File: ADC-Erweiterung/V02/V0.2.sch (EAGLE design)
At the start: 32 parts, among them IC101 ADS124S06IPBS, X101 MOLEX-8738-0343, X102 A97581-ND, X103 A97581-ND, X104 A97581-ND, X105 33PIN-2.54

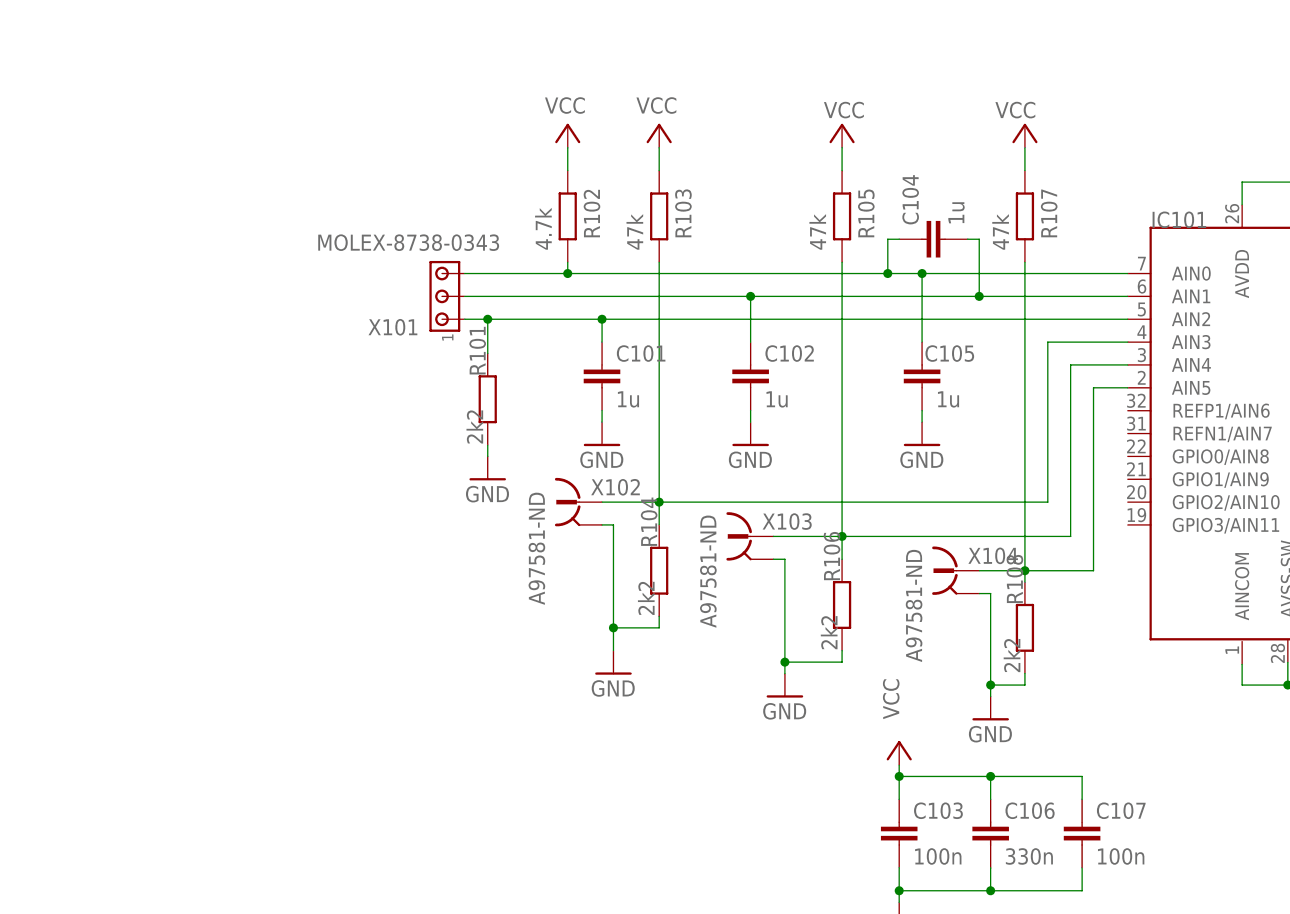
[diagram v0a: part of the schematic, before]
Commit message: AbgabeSoftware
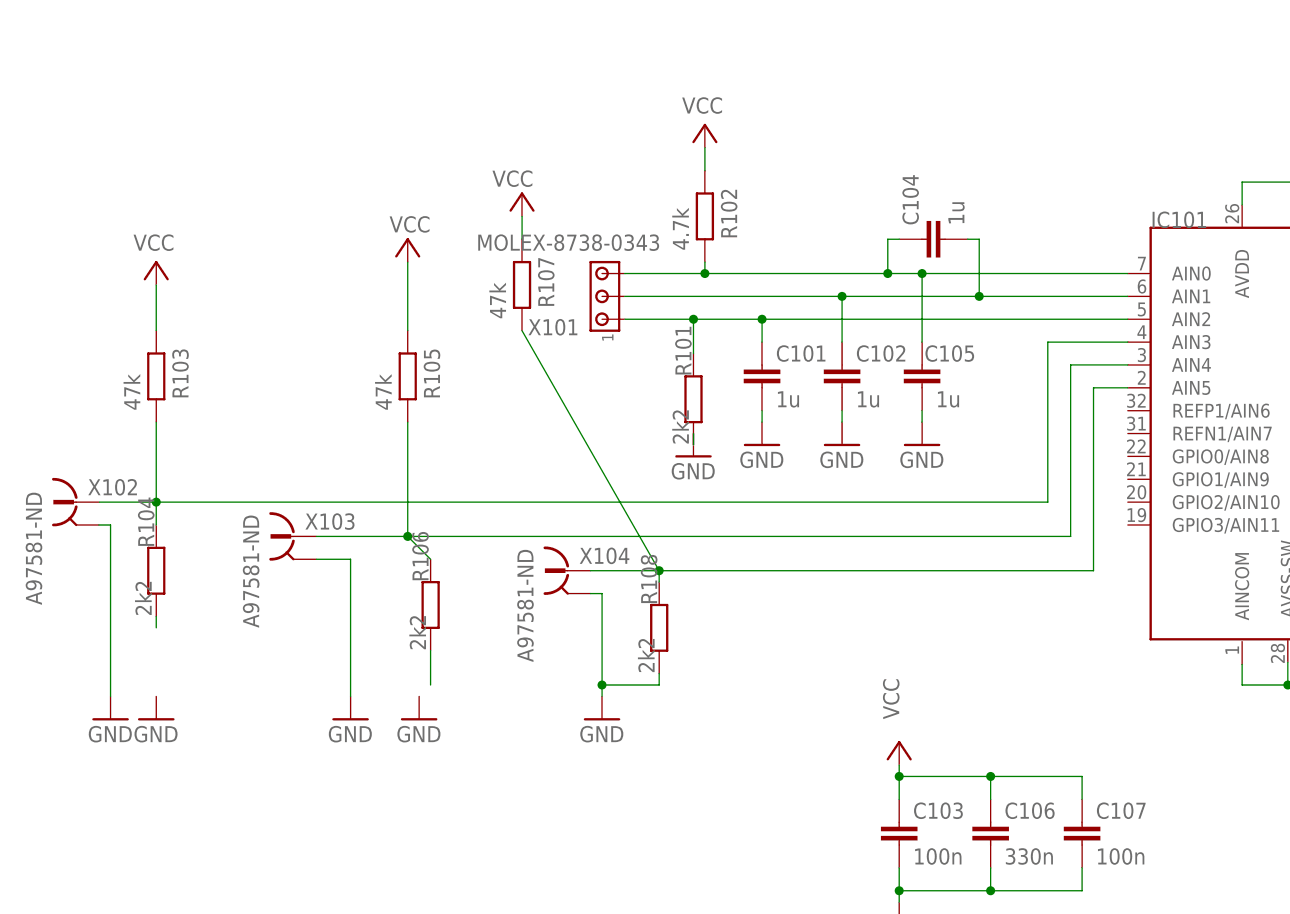
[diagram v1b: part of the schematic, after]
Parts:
- SV101: DIGIKEY_NR (none) -> 732-5321-ND; DIGIKEY_PRICE (none) -> 0.37
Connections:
- new net N$8: R104.1
- new net N$9: R106.1
- net GND: no longer R104.1, R106.1
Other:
- moved on the sheet: C101, C102, R101, R102, R103, R104, R105, R106, R107, R108, X101, X102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

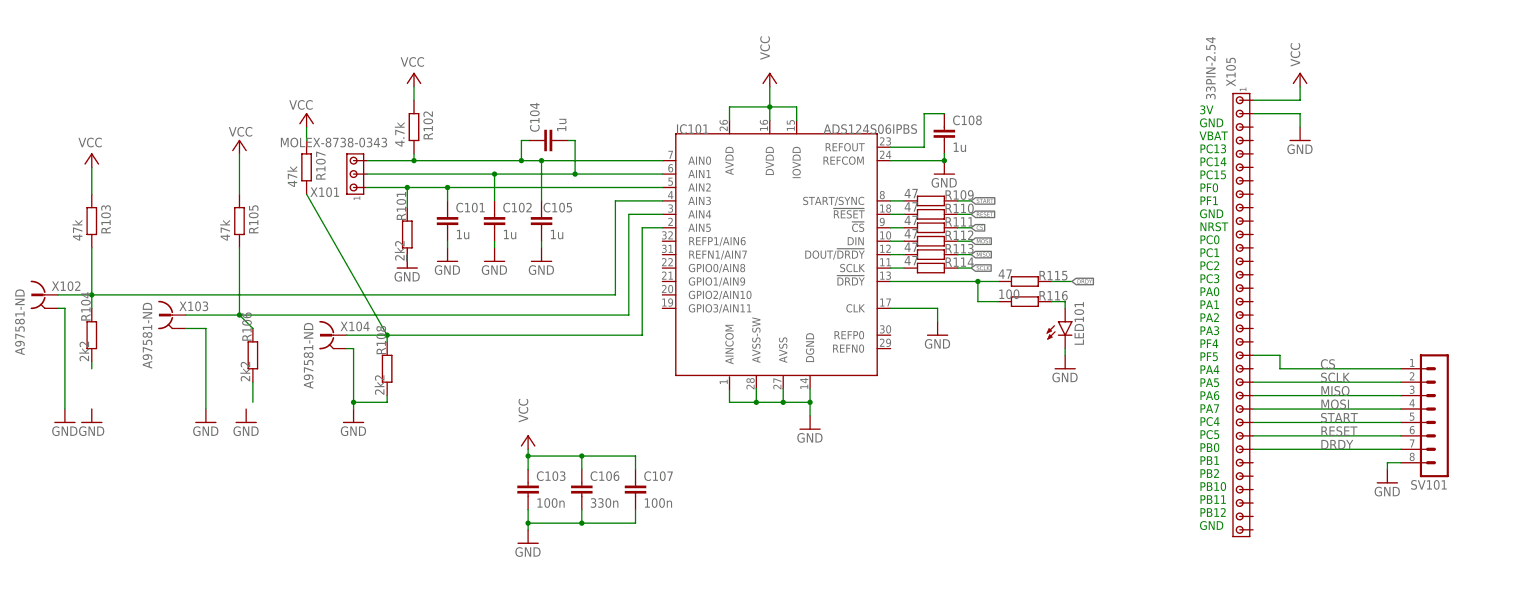
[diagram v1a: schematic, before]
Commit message: improuveschematic
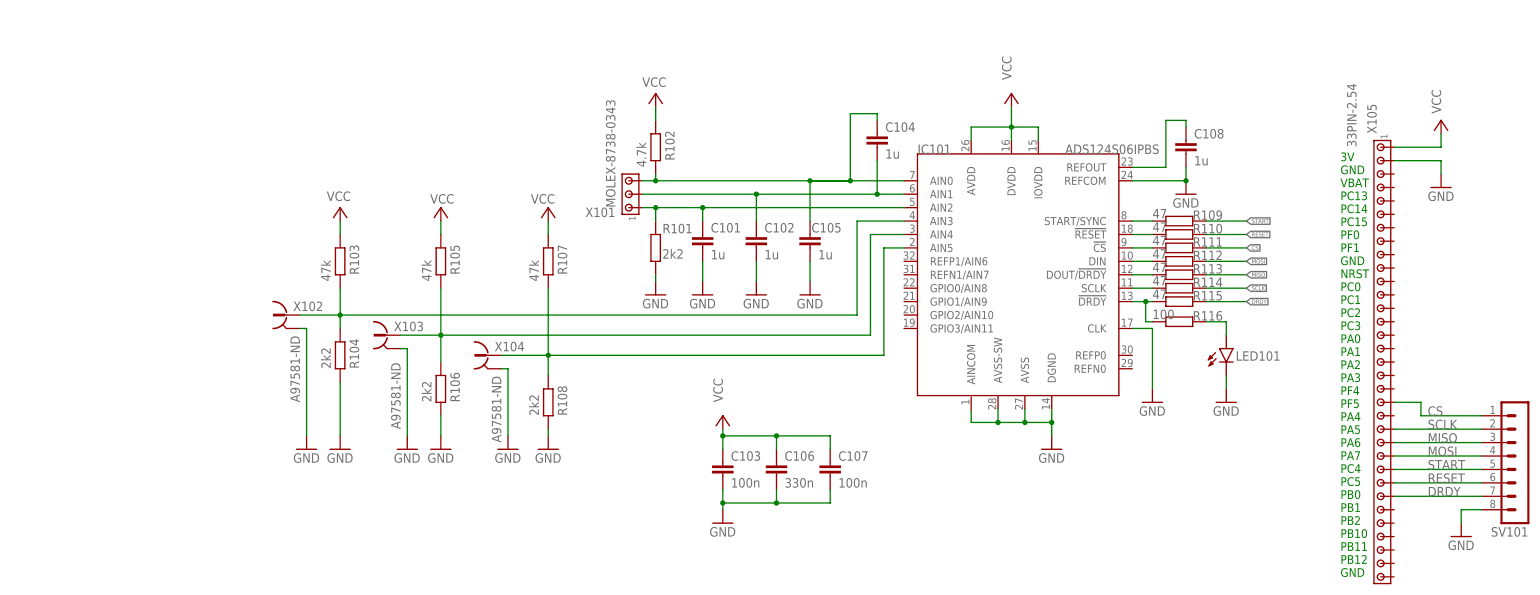
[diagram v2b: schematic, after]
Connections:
- removed net N$8: R104.1
- removed net N$9: R106.1
- net GND: now also R104.1, R106.1
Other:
- moved on the sheet: C101, C102, C103, C104, C105, C106, C107, C108, IC101, LED101, R101, R102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
